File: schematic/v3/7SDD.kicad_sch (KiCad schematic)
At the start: 6 parts, among them U18 SM420561N, U2 SM420561N, U36 SM420561N, U4 YAAJ_BluePill_Part_Like

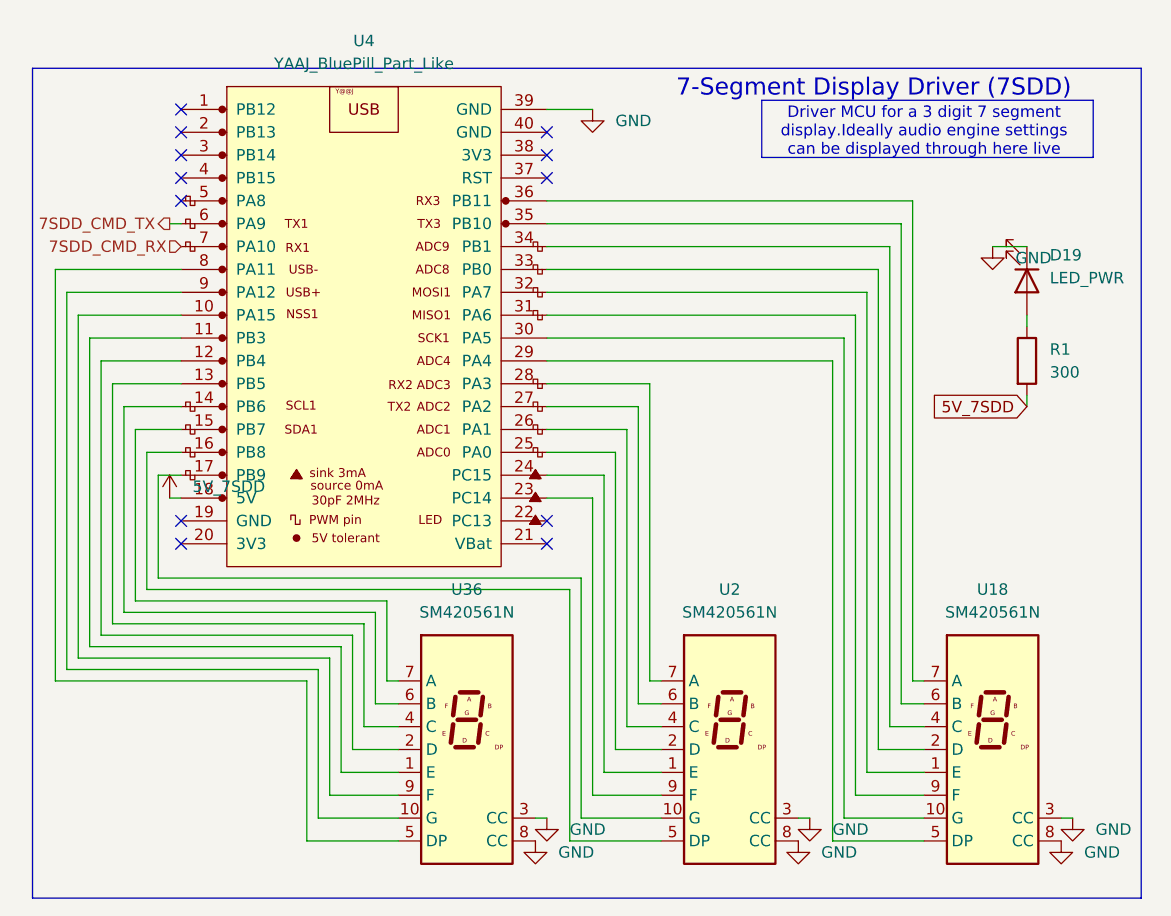
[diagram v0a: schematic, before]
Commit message: progress on creating APM board first
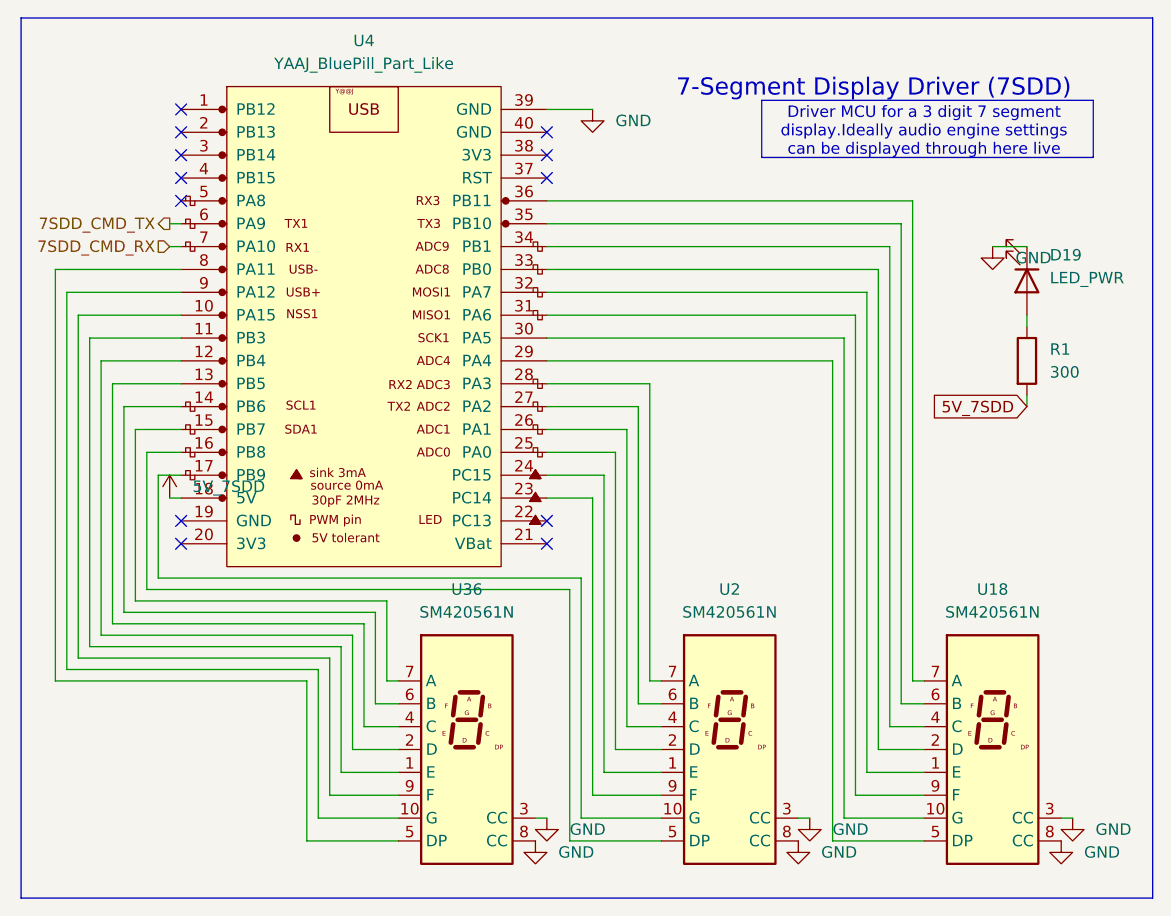
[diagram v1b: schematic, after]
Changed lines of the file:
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@@
 	)
 	(rectangle
-		(start 87.63 55.118)
-		(end 210.82 147.32)
+		(start 86.36 49.53)
+		(end 212.09 147.32)
 		(stroke
 			(width 0)
@@
 		(pts
 			(xy 144.78 69.85) (xy 185.42 69.85)
+		)
+		(stroke
+			(width 0)
+			(type default)
+		)
+	)
+	(wire
+		(pts
+			(xy 102.87 74.93) (xy 104.14 74.93)
 		)
 		(stroke
@@
 	(hierarchical_label "7SDD_CMD_RX"
 		(shape input)
-		(at 104.14 74.93 180)
+		(at 102.87 74.93 180)
 		(effects
 			(font
